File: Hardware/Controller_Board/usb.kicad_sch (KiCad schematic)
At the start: 1 part

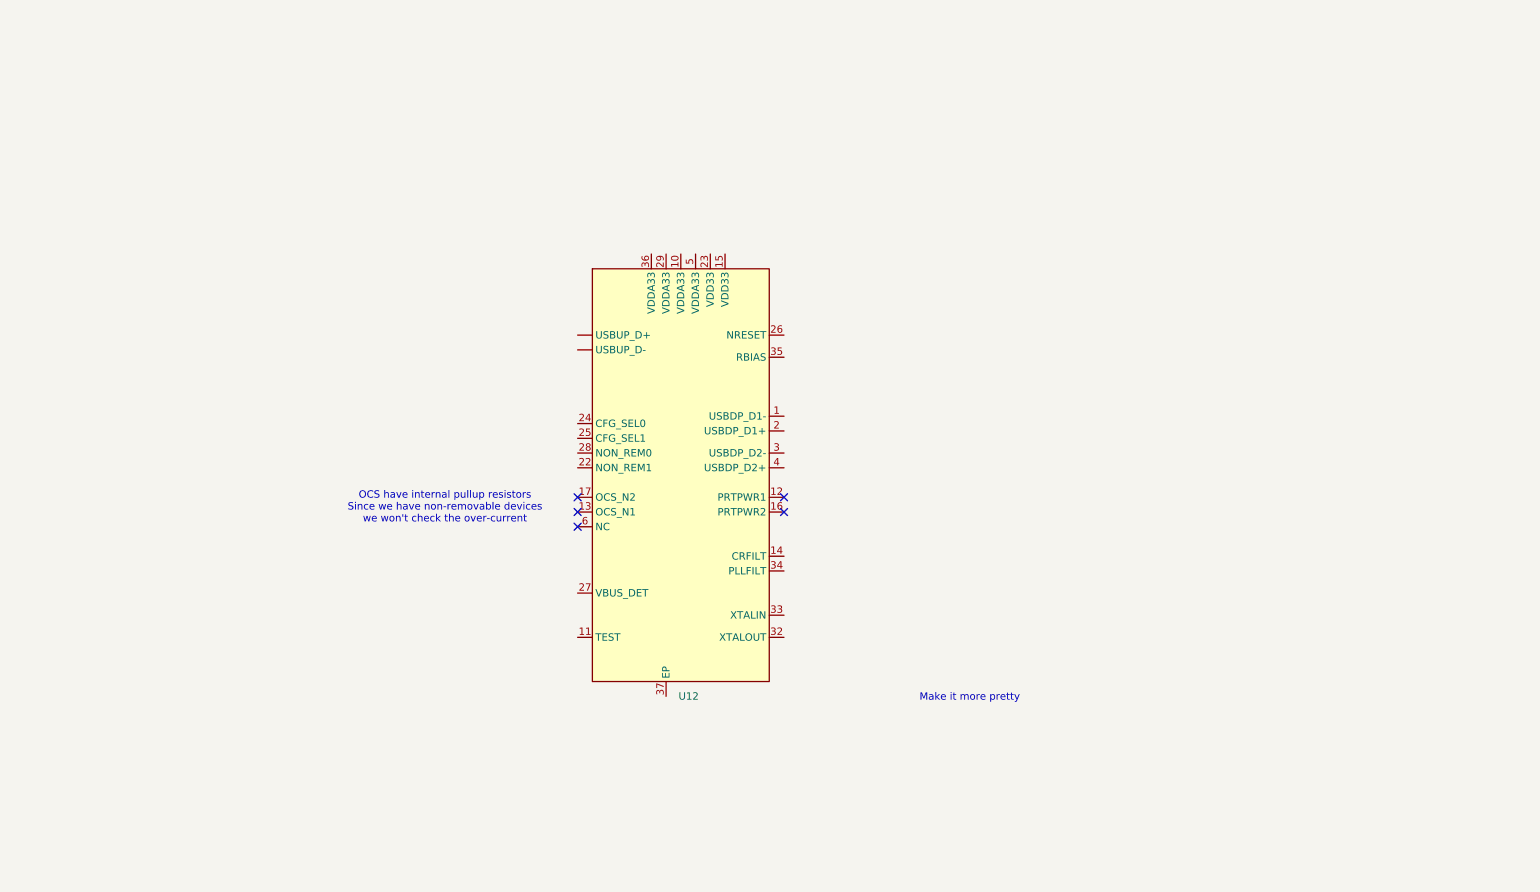
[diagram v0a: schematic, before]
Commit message: Updated the schematic design - Fix the XC7A35T-CPG236 outline issue
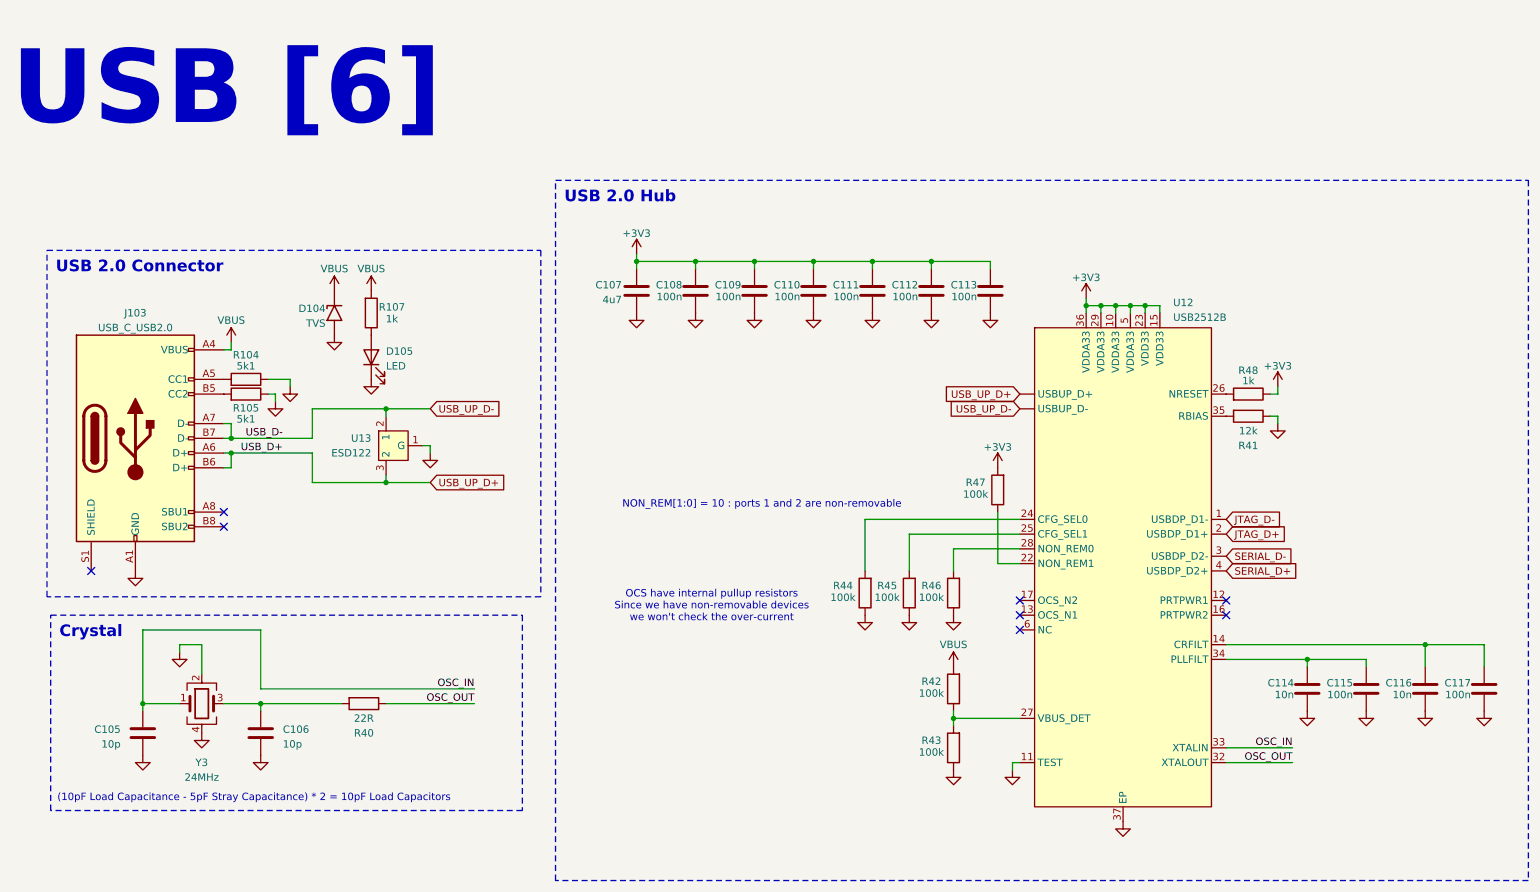
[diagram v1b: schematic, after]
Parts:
- added C105, C106: 10p, Capacitor_SMD:C_0402_1005Metric, symbol Device:C
- added C107: 4u7, Capacitor_SMD:C_0402_1005Metric, symbol Device:C
- added C108, C109, C110, C111, C112, C113, C115, C117: 100n, Capacitor_SMD:C_0402_1005Metric, symbol Device:C
- added C114, C116: 10n, Capacitor_SMD:C_0402_1005Metric, symbol Device:C
- added D104: TVS, Diode_SMD:D_0402_1005Metric, symbol Diode:1.5KExxA
- added D105: LED, LED_SMD:LED_0603_1608Metric, symbol Device:LED
- added J103: USB_C_USB2.0, Connector_USB:USB_C_Receptacle_GCT_USB4105-xx-A_16P_TopMnt_Horizontal, symbol Connector:USB_C_Receptacle_USB2.0
- added R104, R105: 5k1, Resistor_SMD:R_0402_1005Metric, symbol Device:R
- added R107, R48: 1k, Resistor_SMD:R_0402_1005Metric, symbol Device:R
- added R40: 22R, Resistor_SMD:R_0402_1005Metric, symbol Device:R
- added R41: 12k, Resistor_SMD:R_0402_1005Metric, symbol Device:R
- added R42, R43, R44, R45, R46, R47: 100k, Resistor_SMD:R_0402_1005Metric, symbol Device:R
- added U13: ESD122, symbol Custom_VoxLink_Symbols:ESD122
- added Y3: 24MHz, Crystal:Crystal_SMD_2520-4Pin_2.5x2.0mm, symbol Device:Crystal_GND24
- U12: value ~ -> USB2512B
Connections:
- net USB_UP_D-: now reaches U12. (USBUP_D-)
- net USB_UP_D-: now also J103.A7 (D-), J103.B7 (D-), U13.2 (1)
- net JTAG_D-: now reaches U12.1 (USBDP_D1-)
- net +3V3: now reaches U12.10 (VDDA33)
- net +3V3: now also U12.15 (VDD33), U12.23 (VDD33), U12.29 (VDDA33), U12.36 (VDDA33), U12.5 (VDDA33), C107.1, C108.1, C109.1, C110.1, C111.1, C112.1, C113.1, R47.2, R48.1
- net GND: now reaches U12.11 (TEST)
- net GND: now also U12.37 (EP), C105.2, C106.2, C107.2, C108.2, C109.2, C110.2, C111.2, C112.2, C113.2, C114.2, C115.2, C116.2, C117.2, D104.2 (A2), D105.1 (K), J103.A1 (GND), J103.A12 (GND), J103.B1 (GND), J103.B12 (GND), R104.1, R105.1, R41.1, R43.1, R44.1, R45.1, R46.1, U13.1 (G), Y3.2, Y3.4
- net at U12.14 (CRFILT): now also C116.1, C117.1
- net JTAG_D+: now reaches U12.2 (USBDP_D1+)
- net at U12.22 (NON_REM1): now also R47.1
- net at U12.24 (CFG_SEL0): now also R44.2
- net at U12.25 (CFG_SEL1): now also R45.2
- net at U12.26 (NRESET): now also R48.2
- net at U12.27 (VBUS_DET): now also R42.1, R43.2
- net at U12.28 (NON_REM0): now also R46.2
- net SERIAL_D-: now reaches U12.3 (USBDP_D2-)
- net OSC_OUT: now reaches U12.32 (XTALOUT)
- net OSC_OUT: now also R40.1
- net OSC_IN: now reaches U12.33 (XTALIN)
- net OSC_IN: now also C105.1, Y3.1
- net at U12.34 (PLLFILT): now also C114.1, C115.1
- net at U12.35 (RBIAS): now also R41.2
- net SERIAL_D+: now reaches U12.4 (USBDP_D2+)
- new net: D105.2 (A), R107.1
- new net: C106.1, R40.2, Y3.3
- new net: J103.A5 (CC1), R104.2
- new net: J103.B5 (CC2), R105.2
- new net USB_UP_D+: J103.A6 (D+), J103.B6 (D+), U12. (USBUP_D-), U13.3 (2)
- new net VBUS: D104.1 (A1), J103.A4 (VBUS), J103.A9 (VBUS), J103.B4 (VBUS), J103.B9 (VBUS), R107.2, R42.2
- no-connect marks 5 -> 8
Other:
- note added: "(10pF Load Capacitance - 5pF Stray Capacitance) * 2 = 10pF Load Capacitors"
- note added: "NON_REM[1:0] = 10 : ports 1 and 2 are non-removable"
- note added: "USB [6]"
- note removed: "Make it more pretty"

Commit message: Finished schematic design - preparation for review
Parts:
- D104: footprint Diode_SMD:D_0402_1005Metric -> Diode_THT:D_DO-201AE_P15.24mm_Horizontal
